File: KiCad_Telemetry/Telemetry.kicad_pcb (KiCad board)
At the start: 2 copper layers, 67 x 51 mm, 37 parts, among them IC1 TCAN1044VDRQ1, J2 Conn_01x03, J3 PinHeader_01x02, J4 PinHeader_01x02, J7 DB9_Female, J8 USB Micro Connector, U1 NRF24L01_Breakout, U2 STM32F042C4T6, U3 TLV70033_SOT23-5, U4 MCP2518FDT, Y1 Crystal_GND24

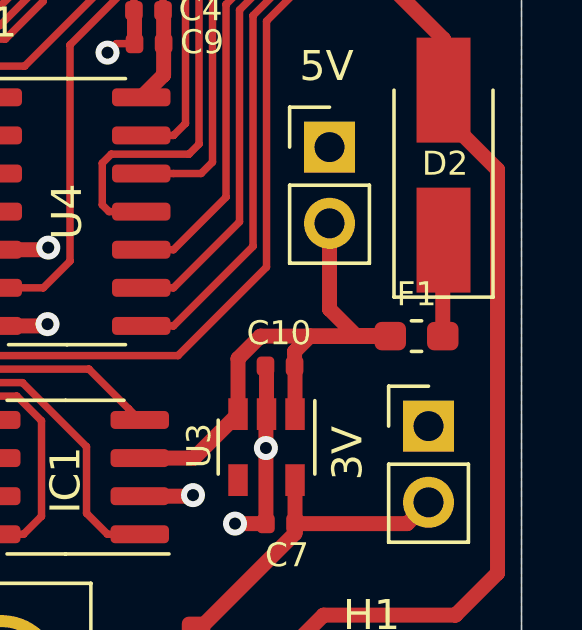
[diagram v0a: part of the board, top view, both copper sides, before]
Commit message: Minor edits; Generated gerber files
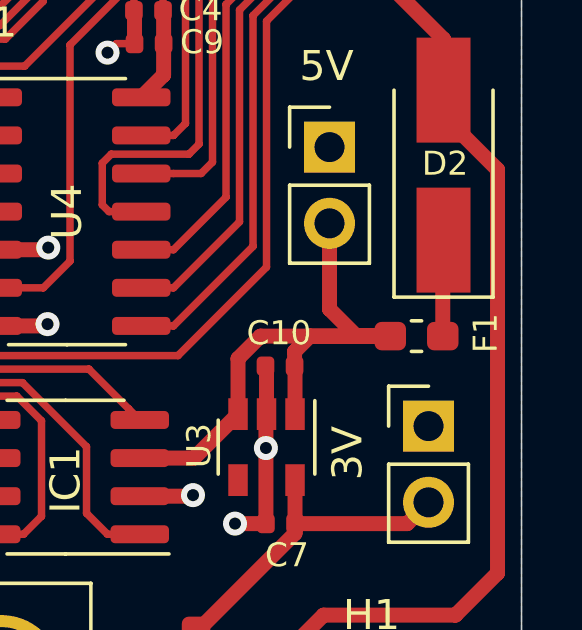
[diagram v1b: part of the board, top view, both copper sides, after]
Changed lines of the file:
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@@
     (0 F.Cu signal)
     (31 B.Cu signal)
-    (32 B.Adhes user)
-    (33 F.Adhes user)
-    (34 B.Paste user)
-    (35 F.Paste user)
+    (32 B.Adhes user hide)
+    (33 F.Adhes user hide)
+    (34 B.Paste user hide)
+    (35 F.Paste user hide)
     (36 B.SilkS user)
     (37 F.SilkS user)
-    (38 B.Mask user)
-    (39 F.Mask user)
-    (40 Dwgs.User user)
+    (38 B.Mask user hide)
+    (39 F.Mask user hide)
+    (40 Dwgs.User user hide)
     (41 Cmts.User user)
     (42 Eco1.User user)
     (43 Eco2.User user)
     (44 Edge.Cuts user)
-    (45 Margin user)
+    (45 Margin user hide)
     (46 B.CrtYd user)
     (47 F.CrtYd user)
-    (48 B.Fab user)
-    (49 F.Fab user)
+    (48 B.Fab user hide)
+    (49 F.Fab user hide)
   )
   (setup
@@
     (tags "resistor handsolder")
     (attr smd)
-    (fp_text reference F1 (at 0 1.4 180) (layer F.SilkS)
+    (fp_text reference F1 (at -2.3 0.1 270) (layer F.SilkS)
       (effects (font (size 0.8 0.8) (thickness 0.15)))
     )
